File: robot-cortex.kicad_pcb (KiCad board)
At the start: 4 copper layers, 27.5 x 26.9 mm, 91 parts, among them IC1 THVD2410VDRCR, IC2 THVD2410VDRCR, IC3 THVD2410VDRCR, J1 USB4110GFA, M1 THRU_HOLE_PAD, M2 THRU_HOLE_PAD, Q1 SS8050-G, Q2 SS8050-G, U1 C2901617, U10 TPS63070, U11 TPS63070, U12 DF52-4S-0.8H(21), U13 DF52-4S-0.8H(21), U14 DF52-4S-0.8H(21), U2 STM32G431CBT6, U3 TLE9250XSJXUMA1, U4 DF52-3S-0.8H(21), U5 DF52-4S-0.8H(21), U6 SPX3819M5-L-5-0, U7 DF52-8S-0.8H(21), U8 ESP32-WROOM-32E-H4, U9 CP2102N-A02-GQFN24R

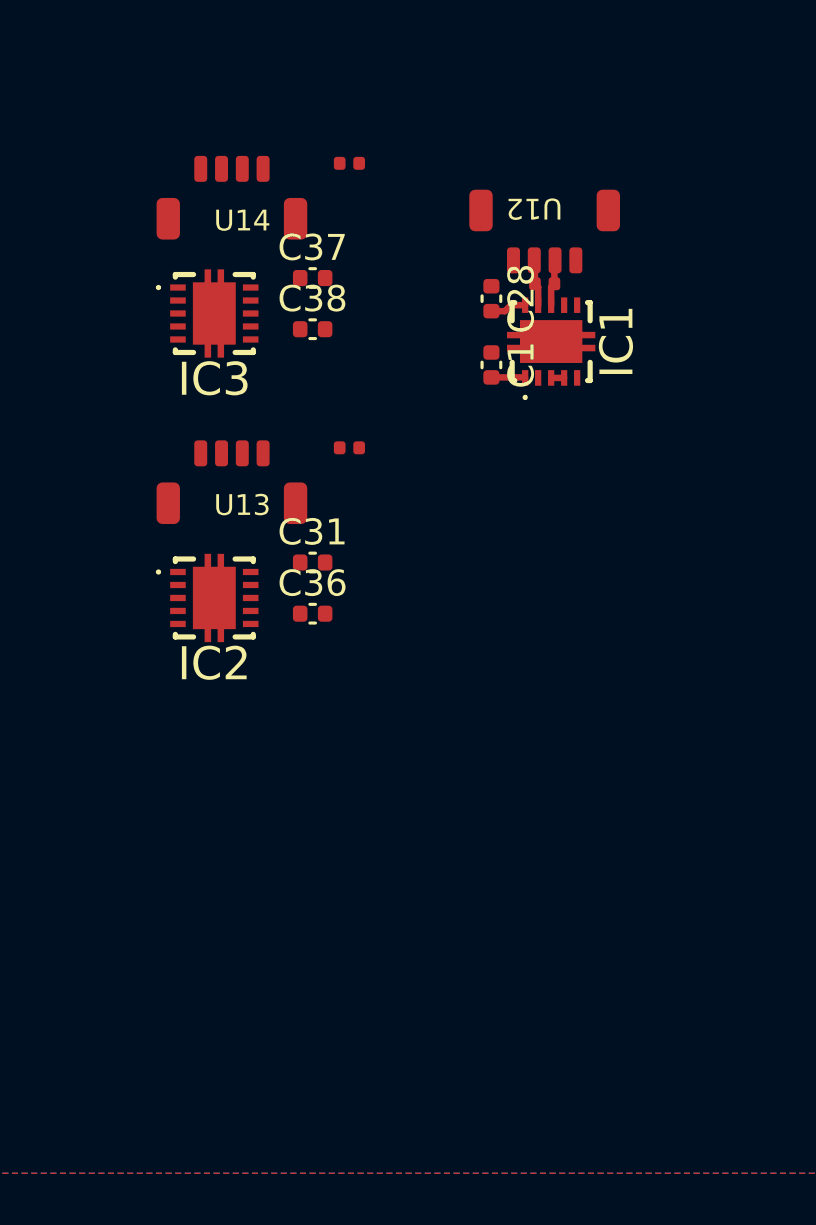
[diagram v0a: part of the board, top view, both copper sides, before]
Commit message: fix vbat
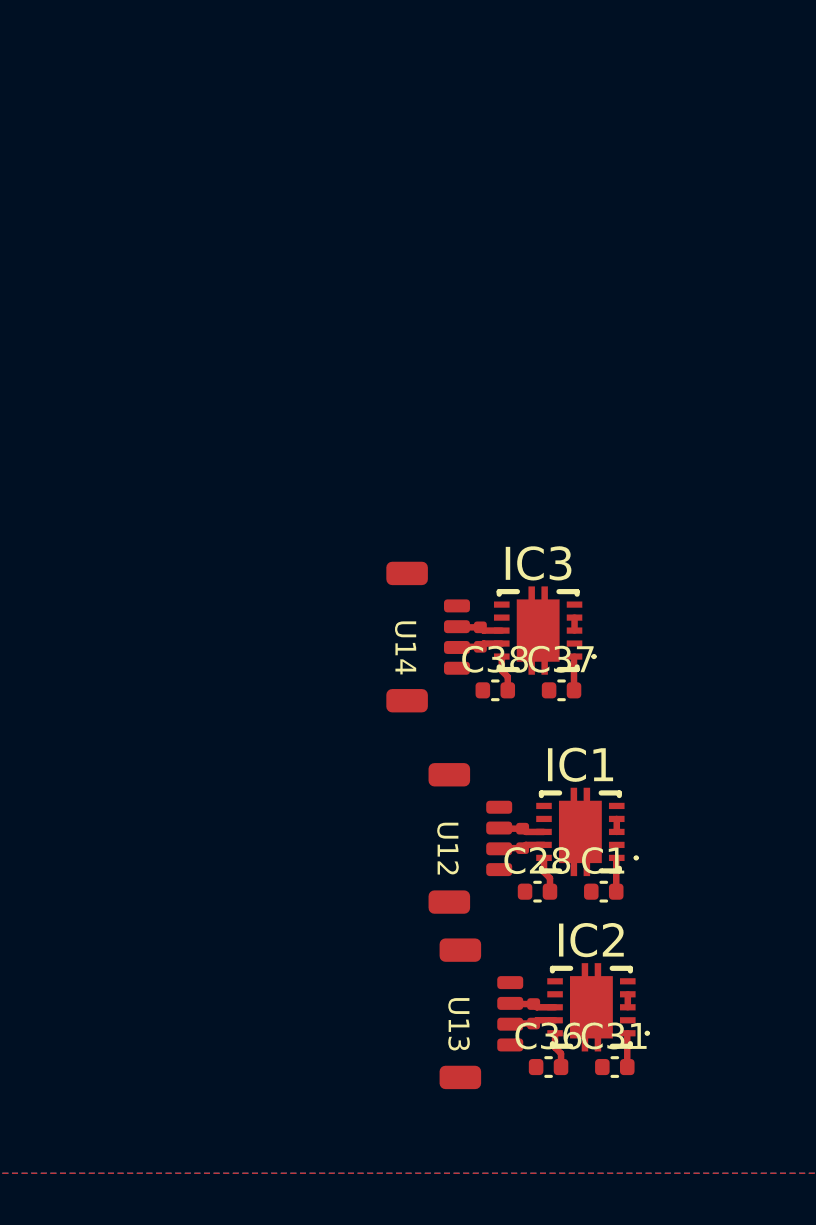
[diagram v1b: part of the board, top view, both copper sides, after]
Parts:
- moved U13 24.1 mm to (175.9, 127.5), turned to -90 degrees
- moved R20 22.9 mm to (176.8, 127.5), turned to -90 degrees
- moved C28 22.9 mm to (176.9, 122.8), turned to 0 degrees
- moved C31 22.6 mm to (179.9, 129.6)
- moved U12 22.3 mm to (175.5, 120.8), turned to -90 degrees
- moved IC2 21.4 mm to (179.0, 127.2), turned to 180 degrees
- moved R19 21.4 mm to (176.4, 120.8), turned to -90 degrees
- moved C1 20.7 mm to (179.5, 122.8), turned to 0 degrees
- moved U14 20.0 mm to (173.8, 113.0), turned to -90 degrees
- moved C36 19.7 mm to (177.4, 129.6)
- moved R21 18.9 mm to (174.8, 113.0), turned to -90 degrees
- moved IC1 18.9 mm to (178.6, 120.5), turned to 180 degrees
- moved C37 18.5 mm to (177.9, 115.0)
- moved IC3 17.4 mm to (177.0, 112.8), turned to 180 degrees
- moved C38 15.6 mm to (175.3, 115.0)
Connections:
- U12 pad 1: /RS485 Transceiver/VBAT -> /VBAT
- U13 pad 1: /RS485 Transceiver1/VBAT -> /VBAT
- U14 pad 1: /RS485 Transceiver2/VBAT -> /VBAT
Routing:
- net /+5V0: track 46.2 -> 49.0 mm
- net +3V3: track 52.3 -> 54.9 mm
- net /RS485 Transceiver2/RS1_B: track 0.00 -> 1.79 mm
- net /RS485 Transceiver2/RS1_A: track 0.00 -> 1.79 mm
- net /RS485 Transceiver1/RS1_B: track 0.00 -> 1.79 mm
- net /RS485 Transceiver1/RS1_A: track 0.00 -> 1.79 mm
- net /USART3_DE: track 0.00 -> 0.50 mm
- net /USART2_DE: track 0.00 -> 0.50 mm
